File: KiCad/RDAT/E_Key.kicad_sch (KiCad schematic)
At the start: 12 parts, among them J16 MDT420E03001

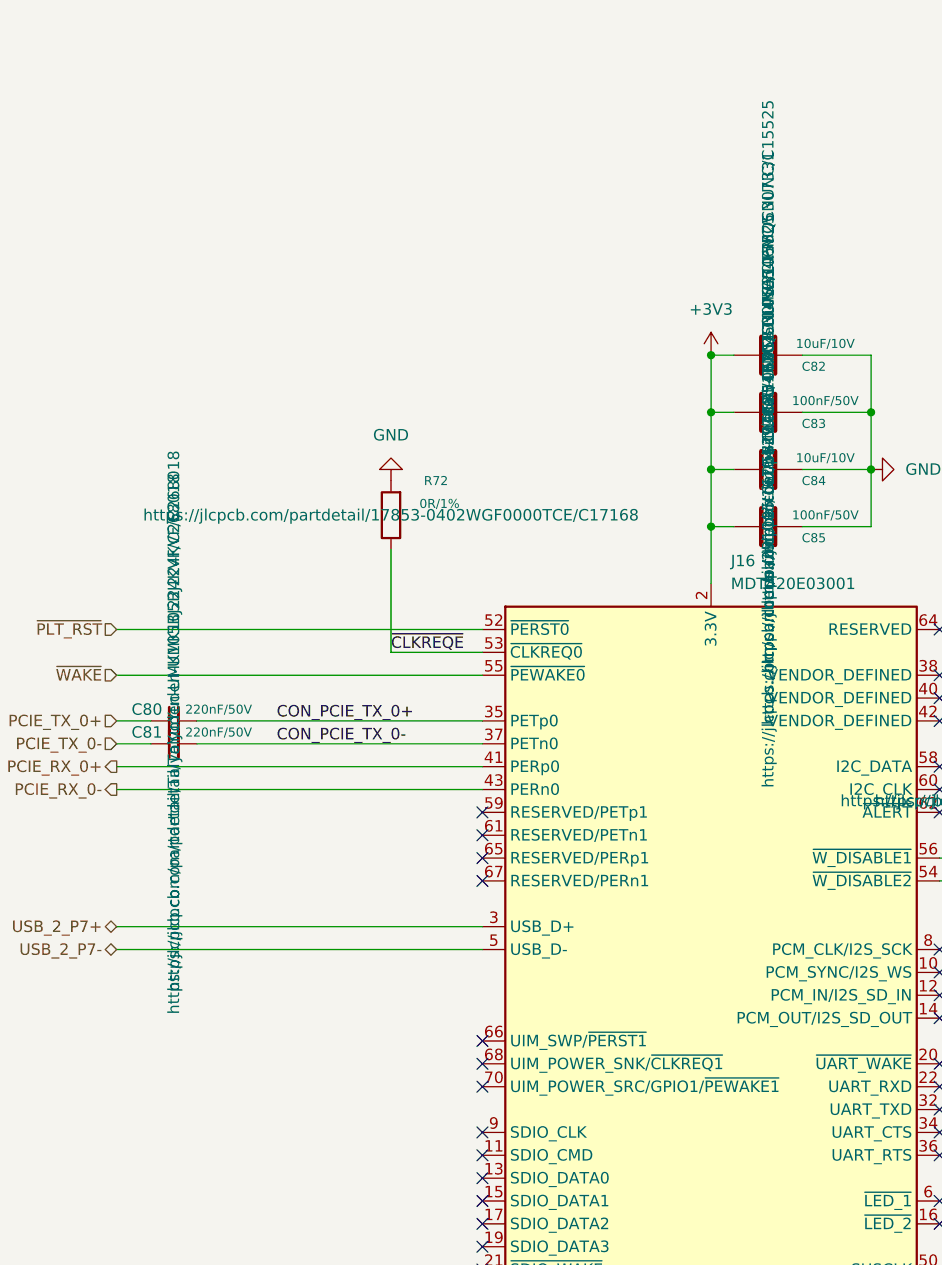
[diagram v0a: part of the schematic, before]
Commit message: Push before Board Layout
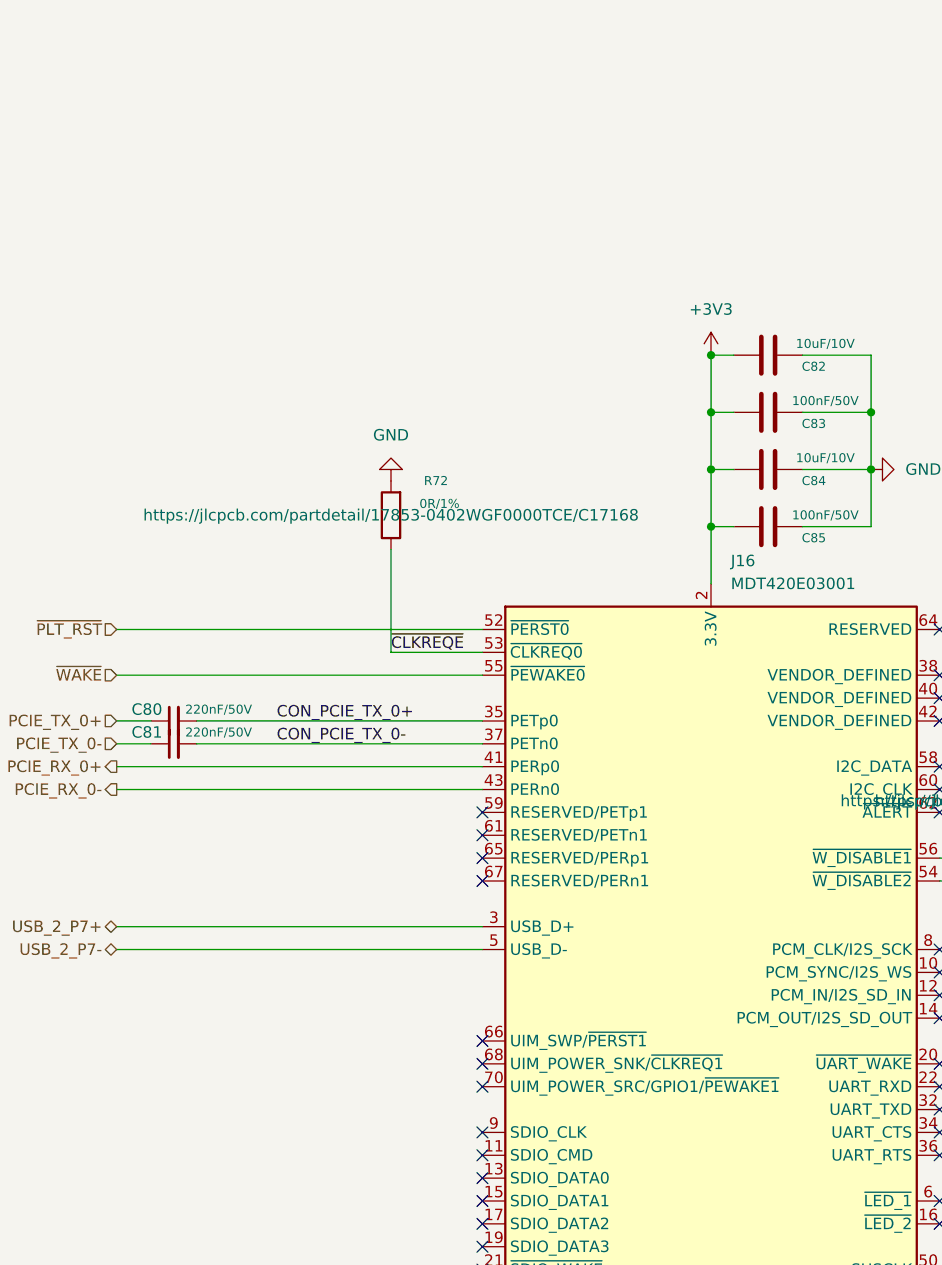
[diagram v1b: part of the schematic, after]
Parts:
- C80, C81, C82, C83, C84, C85: footprint A_HDJ_Library:C_0402_1005Metric -> Capacitor_SMD:C_0402_1005Metric
- H8: footprint A_HDJ_Library:MountingHole_2.75mm_M2_4.4mm_Pad_TopOnly -> MountingHole:MountingHole_2.2mm_M2_Pad_TopBottom
- R72, R73, R74, R75: footprint A_HDJ_Library:R_0402_1005Metric -> Resistor_SMD:R_0402_1005Metric
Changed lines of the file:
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@@
 			)
 		)
-		(property "Footprint" "A_HDJ_Library:C_0402_1005Metric"
+		(property "Footprint" "Capacitor_SMD:C_0402_1005Metric"
 			(at 77.47 85.09 0)
 			(effects
@@
 					(size 1.27 1.27)
 				)
+				(hide yes)
 			)
 		)
@@
 			)
 		)
-		(property "Footprint" "A_HDJ_Library:C_0402_1005Metric"
+		(property "Footprint" "Capacitor_SMD:C_0402_1005Metric"
 			(at 77.47 87.63 0)
 			(effects
@@
 					(size 1.27 1.27)
 				)
+				(hide yes)
 			)
 		)
@@
 			)
 		)
-		(property "Footprint" "A_HDJ_Library:R_0402_1005Metric"
+		(property "Footprint" "Resistor_SMD:R_0402_1005Metric"
 			(at 180.848 93.98 90)
 			(effects
@@
 			)
 		)
-		(property "Footprint" "A_HDJ_Library:C_0402_1005Metric"
+		(property "Footprint" "Capacitor_SMD:C_0402_1005Metric"
 			(at 139.7 58.1152 0)
 			(effects
@@
 					(size 1.27 1.27)
 				)
+				(hide yes)
 			)
 		)
@@
 			)
 		)
-		(property "Footprint" "A_HDJ_Library:C_0402_1005Metric"
+		(property "Footprint" "Capacitor_SMD:C_0402_1005Metric"
 			(at 139.7 45.4152 0)
 			(effects
@@
 					(size 1.27 1.27)
 				)
+				(hide yes)
 			)
 		)
@@
 			)
 		)
-		(property "Footprint" "A_HDJ_Library:R_0402_1005Metric"
+		(property "Footprint" "Resistor_SMD:R_0402_1005Metric"
 			(at 177.8 147.828 90)
 			(effects
@@
 			)
 		)
-		(property "Footprint" "A_HDJ_Library:R_0402_1005Metric"
+		(property "Footprint" "Resistor_SMD:R_0402_1005Metric"
 			(at 103.378 62.23 90)
 			(effects
@@
 			)
 		)
-		(property "Footprint" "A_HDJ_Library:MountingHole_2.75mm_M2_4.4mm_Pad_TopOnly"
+		(property "Footprint" "MountingHole:MountingHole_2.2mm_M2_Pad_TopBottom"
 			(at 25.4 92.71 0)
 			(effects
@@
 			)
 		)
-		(property "Footprint" "A_HDJ_Library:C_0402_1005Metric"
+		(property "Footprint" "Capacitor_SMD:C_0402_1005Metric"
 			(at 139.7 64.4652 0)
 			(effects
@@
 					(size 1.27 1.27)
 				)
+				(hide yes)
 			)
 		)
@@
 			)
 		)
-		(property "Footprint" "A_HDJ_Library:C_0402_1005Metric"
+		(property "Footprint" "Capacitor_SMD:C_0402_1005Metric"
 			(at 139.7 51.7652 0)
 			(effects
@@
 					(size 1.27 1.27)
 				)
+				(hide yes)
 			)
 		)
@@
 			)
 		)
-		(property "Footprint" "A_HDJ_Library:R_0402_1005Metric"
+		(property "Footprint" "Resistor_SMD:R_0402_1005Metric"
 			(at 181.102 93.98 90)
 			(effects

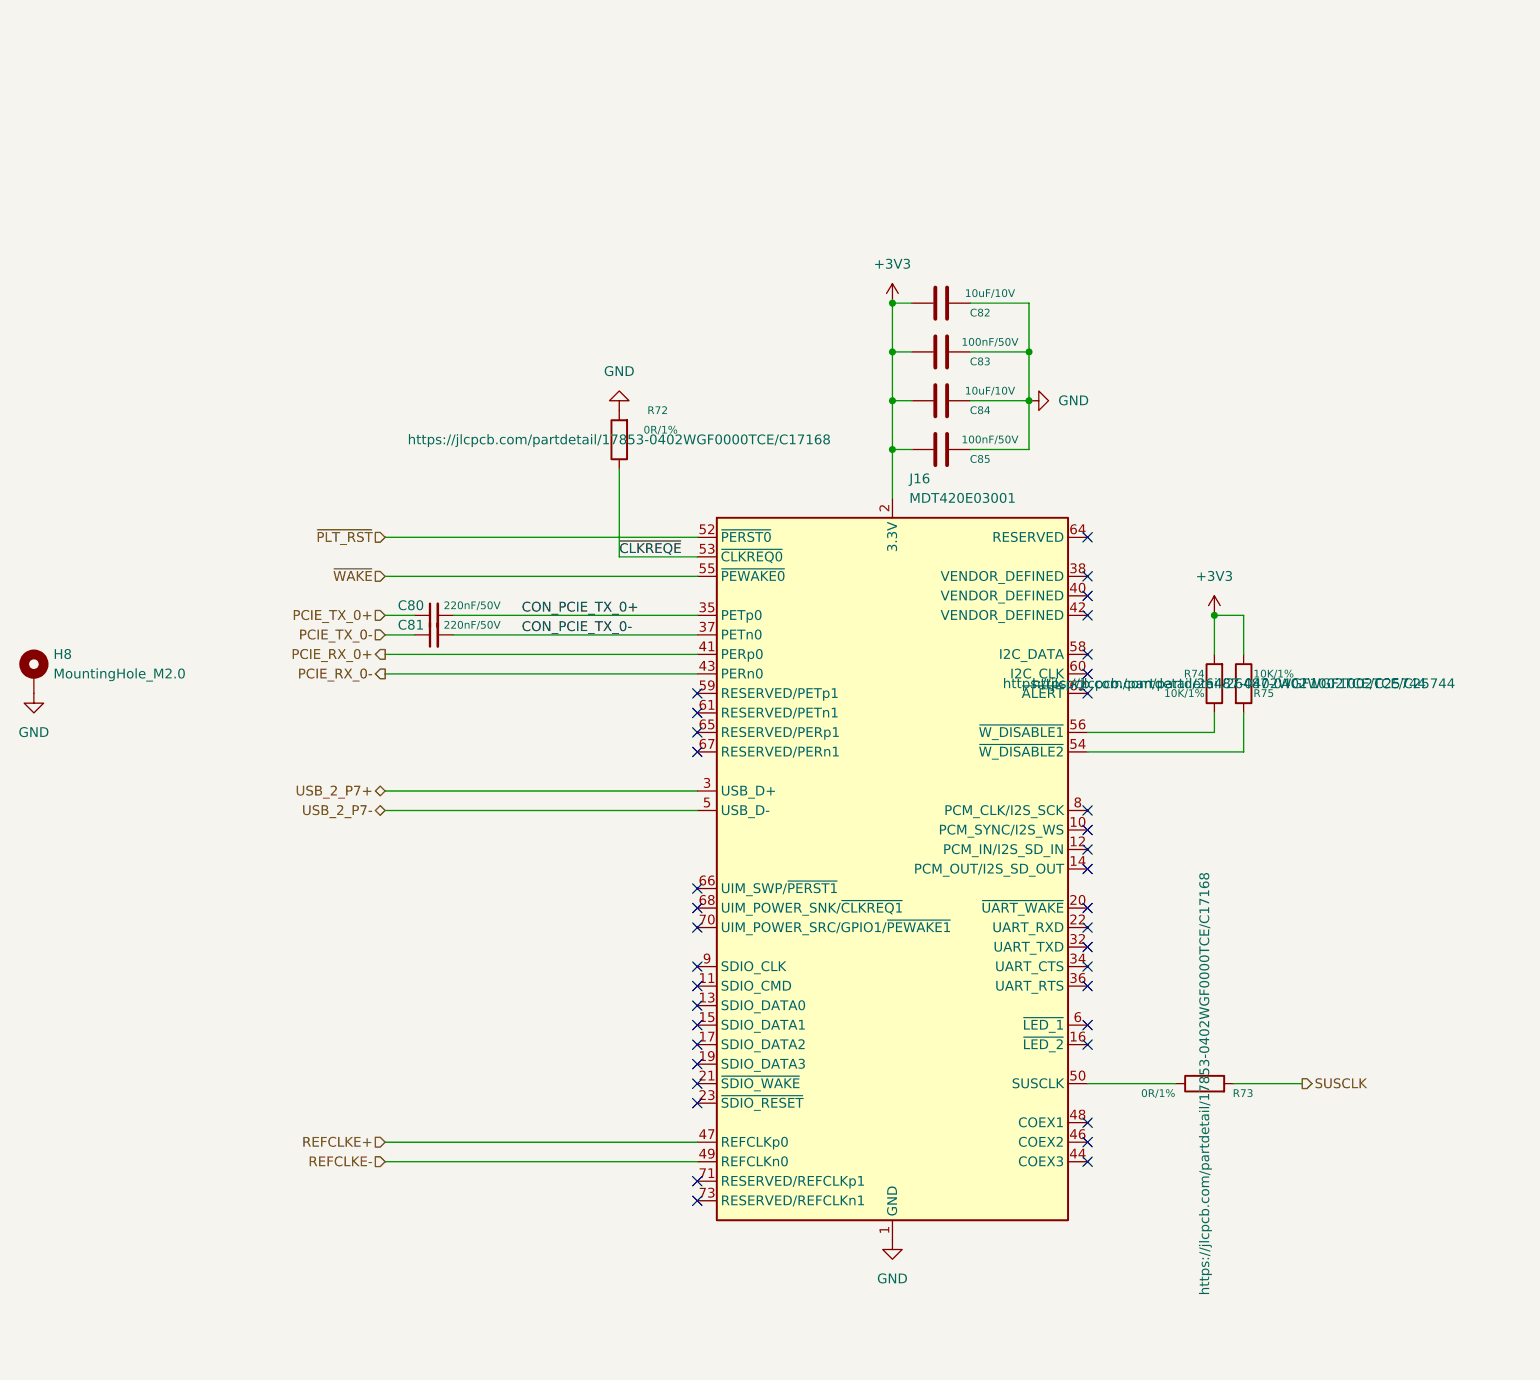
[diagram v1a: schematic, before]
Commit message: Placed a lot of components
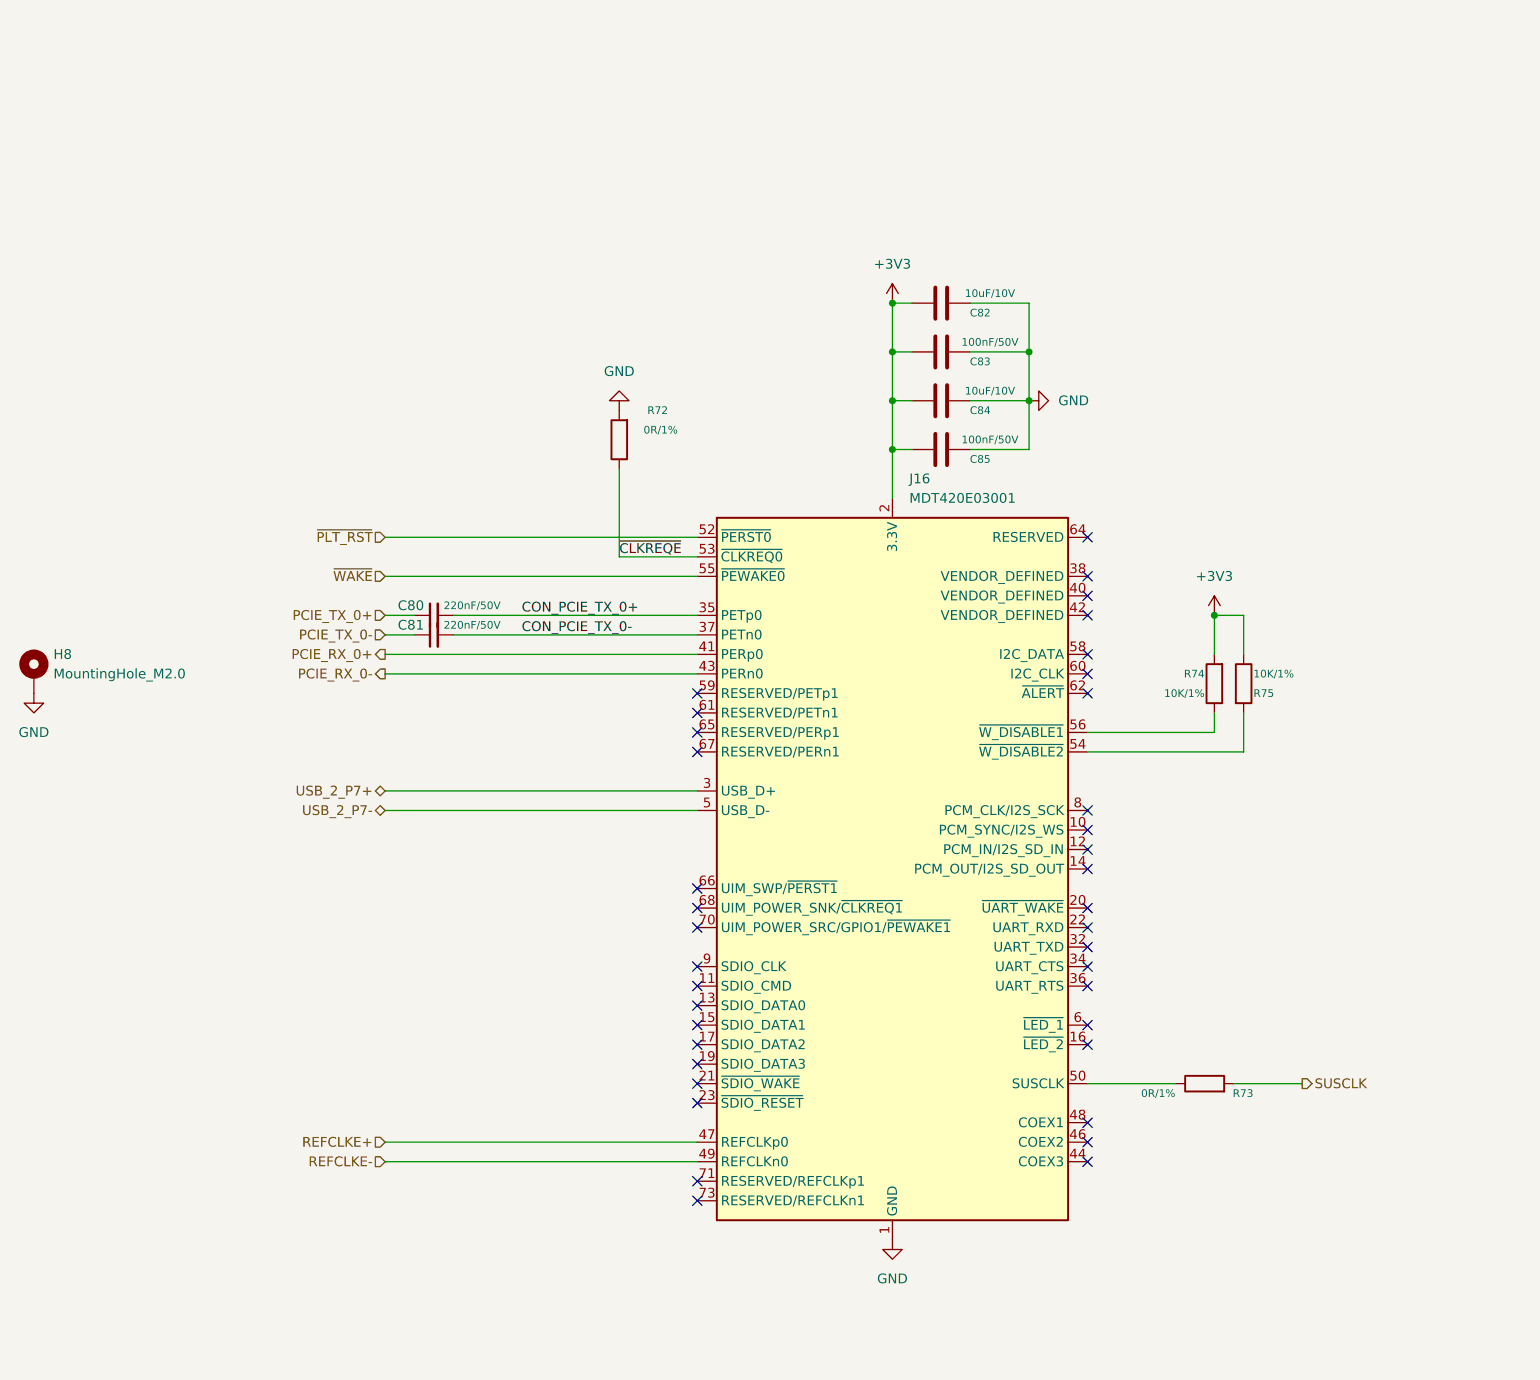
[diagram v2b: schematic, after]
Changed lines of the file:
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@@
 					(size 1.27 1.27)
 				)
+				(hide yes)
 			)
 		)
@@
 					(size 1.27 1.27)
 				)
+				(hide yes)
 			)
 		)
@@
 					(size 1.27 1.27)
 				)
+				(hide yes)
 			)
 		)
@@
 					(size 1.27 1.27)
 				)
-			)
-		)
+				(hide yes)
+			)
+		)
